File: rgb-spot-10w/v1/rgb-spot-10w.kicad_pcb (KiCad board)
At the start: 2 copper layers, 68 x 86.5 mm, 6 parts, among them J1 Conn_01x05_Male, J2 Screw_Terminal_01x02, J3 Conn_02x04_Odd_Even, SW1 SW_DPDT_x2, U1 ESP32-POE-ISO

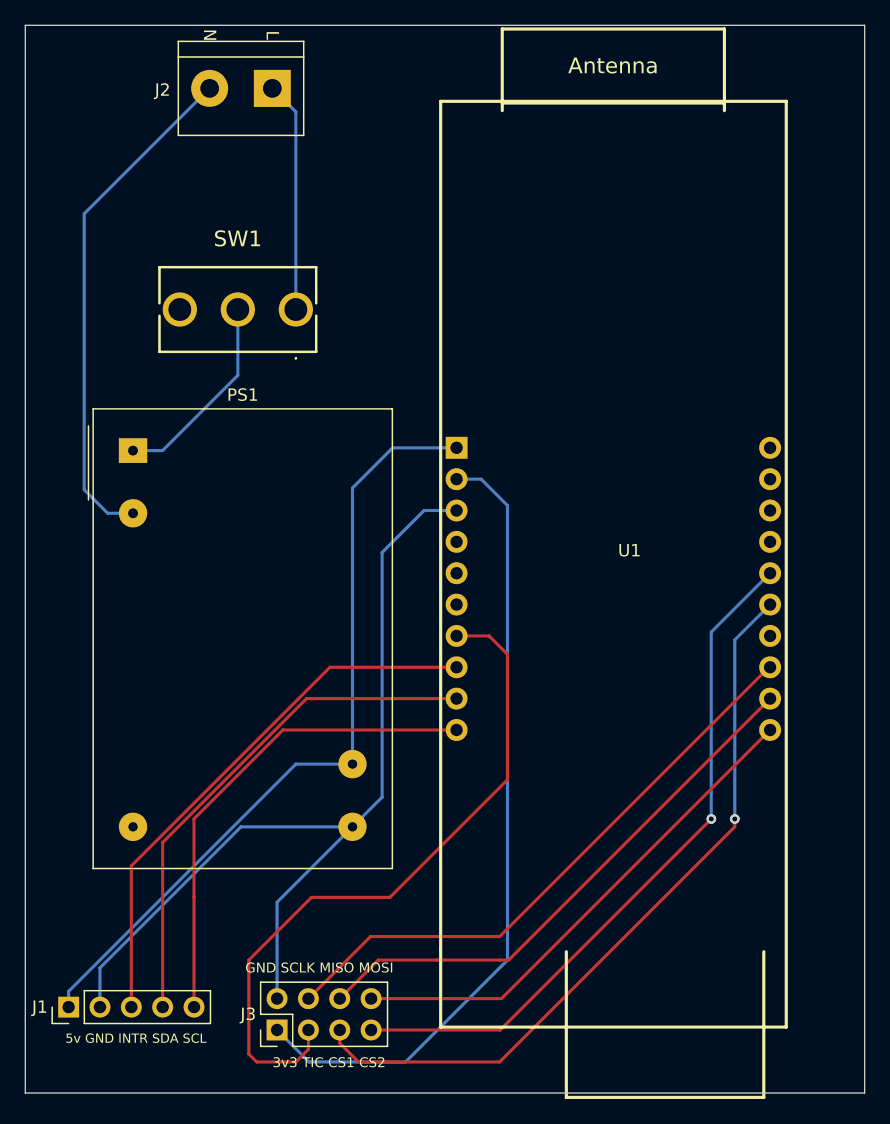
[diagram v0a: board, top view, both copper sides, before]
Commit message: pcb OK
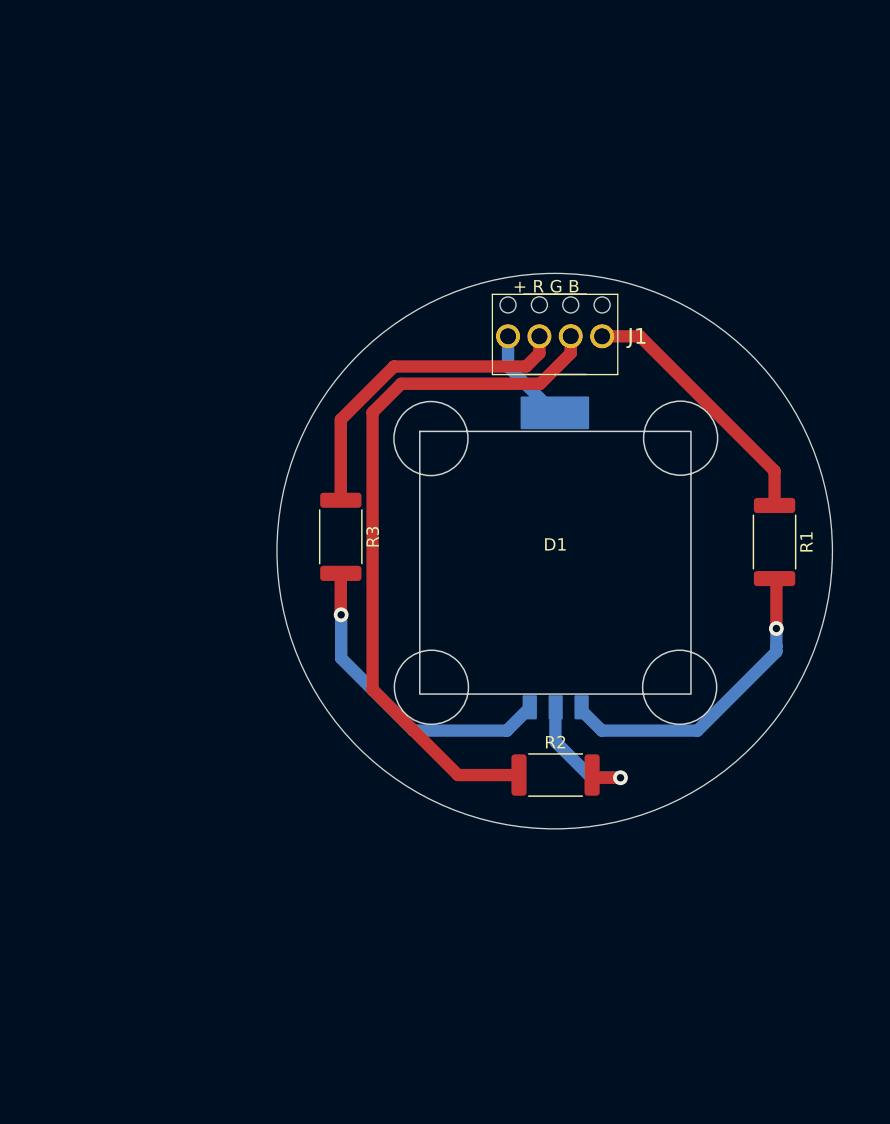
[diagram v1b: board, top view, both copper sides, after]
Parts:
- removed J2: Screw_Terminal_01x02, TerminalBlock:TerminalBlock_bornier-2_P5.08mm
- removed J3: Conn_02x04_Odd_Even, Connector_PinHeader_2.54mm:PinHeader_2x04_P2.54mm_Vertical
- removed PS1: Alim RS PRO 5V 1A, Converter_ACDC:Converter_ACDC_MeanWell_IRM-03-xx_THT
- removed SW1: SW_DPDT_x2, mylife-footprints:RS PRO Switch 401-703
- removed U1: ESP32-POE-ISO, mylife-footprints:ESP32-POE
- added D1: LED_ARGB, mylife-footprints:LED RGB 10W, F.Cu at (142.9, 92.6)
- added R1: 5.1Ω/1W, Resistor_SMD:R_2512_6332Metric, F.Cu at (160.7, 91.9)
- added R2: 5.1Ω/1W, Resistor_SMD:R_2512_6332Metric, F.Cu at (143.0, 110.7)
- added R3: 10Ω/1W, Resistor_SMD:R_2512_6332Metric, F.Cu at (125.6, 91.4)
- J1: value Conn_01x05_Male -> Screw_Terminal_01x04; footprint Connector_PinHeader_2.54mm:PinHeader_1x05_P2.54mm_Vertical -> mylife-footprints:RS PRO Terminal Small x4
- moved J1 69.4 mm to (146.7, 75.2), turned to 180 degrees
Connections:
- J1 pad 1: +5V -> Net-(J1-Pin_1)
- J1 pad 2: GND -> Net-(J1-Pin_2)
- J1 pad 3: /INTR -> Net-(J1-Pin_3)
- J1 pad 4: /SDA -> Net-(D1-A)
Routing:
- net GND: track 75.5 -> 0.00 mm
- net +3V3: track 65.0 -> 0.00 mm
- net +5V: track 64.0 -> 0.00 mm
- net /CS1: track 60.8 -> 0.00 mm, vias 1 -> 0
- net Net-(J1-Pin_2): track 0.00 -> 56.6 mm
- net /TIC: track 56.6 -> 0.00 mm
- net /CS2: track 56.5 -> 0.00 mm, vias 1 -> 0
- net /SCLK: track 48.5 -> 0.00 mm
- net /MISO: track 44.9 -> 0.00 mm
- net /INTR: track 44.5 -> 0.00 mm
- net /SDA: track 42.0 -> 0.00 mm
- net NEUT: track 41.5 -> 0.00 mm
- net /MOSI: track 41.3 -> 0.00 mm
- net /SCL: track 39.5 -> 0.00 mm
- net Net-(J1-Pin_3): track 0.00 -> 26.2 mm
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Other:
- board size 68 x 86.5 mm -> 45 x 45 mm
- board text added: "+ R G B"
- board text removed: "3v3 TIC CS1 CS2"
- board text removed: "5v GND INTR SDA SCL"
- board text removed: "GND SCLK MISO MOSI"
- board text removed: "L"
- board text removed: "N"
